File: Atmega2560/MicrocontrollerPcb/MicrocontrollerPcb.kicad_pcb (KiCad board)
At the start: 2 copper layers, 65.4 x 46.4 mm, 47 parts, among them J1 Conn_02x12_Odd_Even, J2 USB_B_Micro, U1 ATmega2560-16AU, U2 ATmega8U2-MU

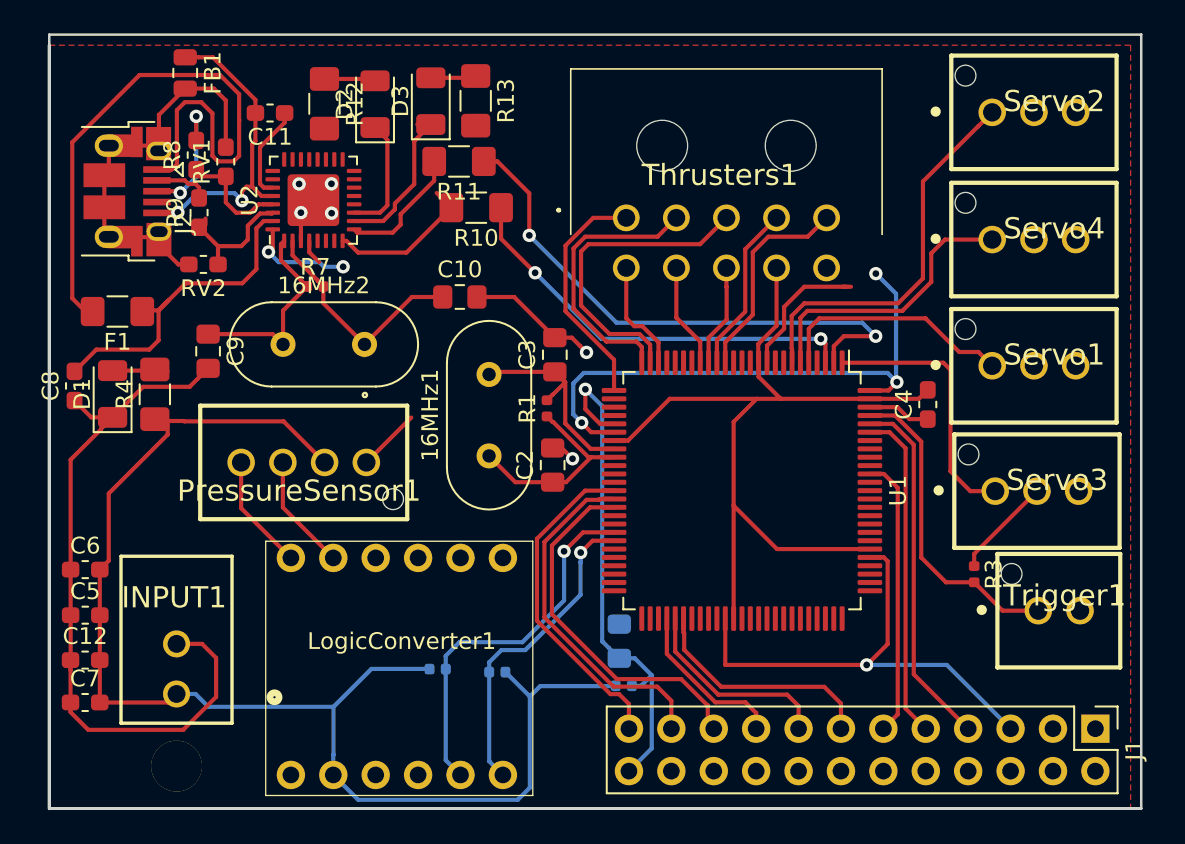
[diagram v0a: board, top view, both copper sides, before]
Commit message: Added Gerber Files
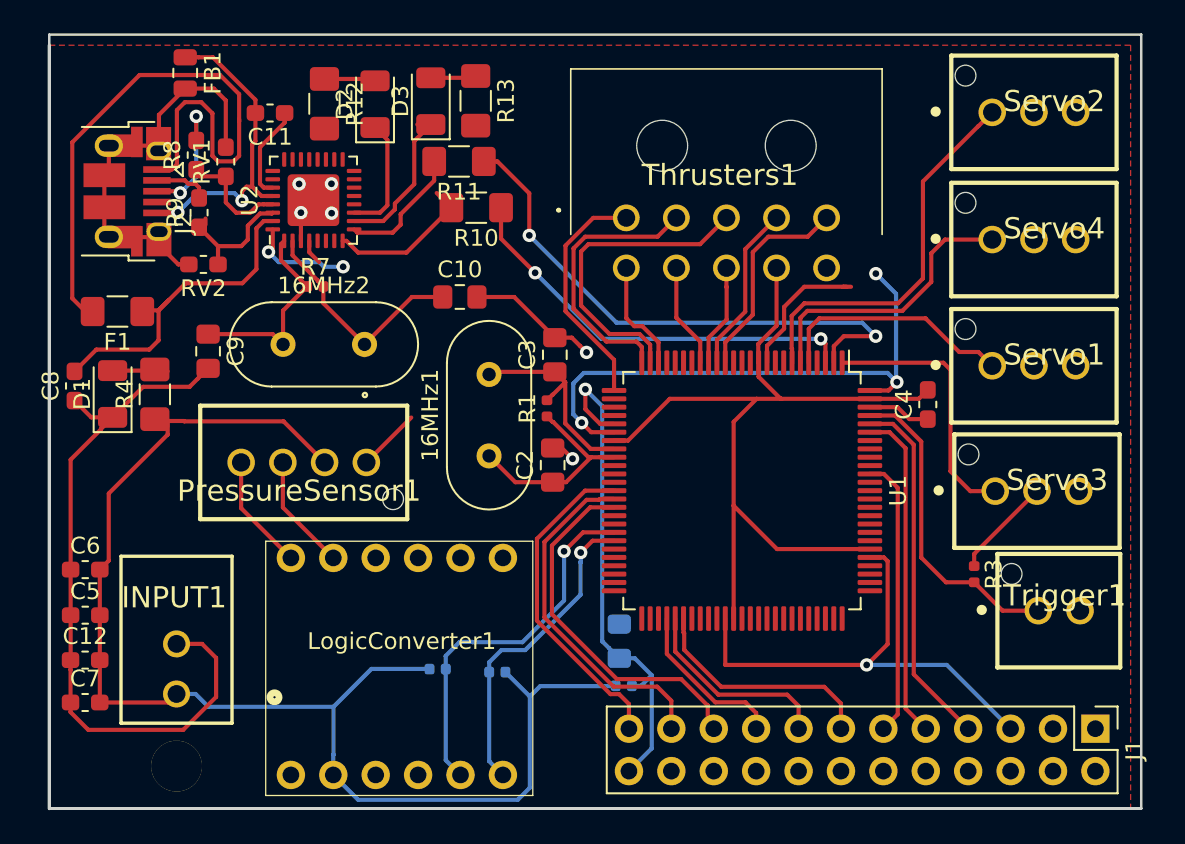
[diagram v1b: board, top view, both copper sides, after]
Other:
- net class Default removed
